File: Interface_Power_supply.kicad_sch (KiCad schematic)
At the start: 0 parts

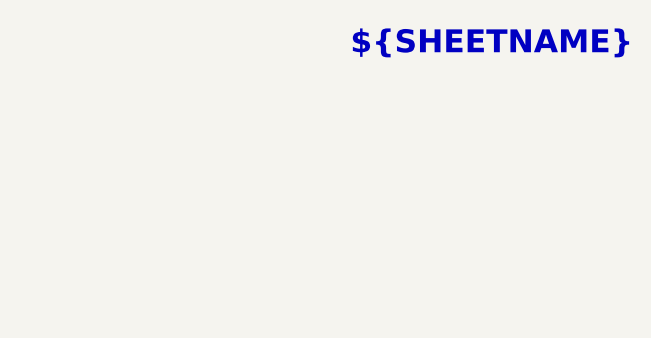
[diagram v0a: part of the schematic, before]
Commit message: testing green mask
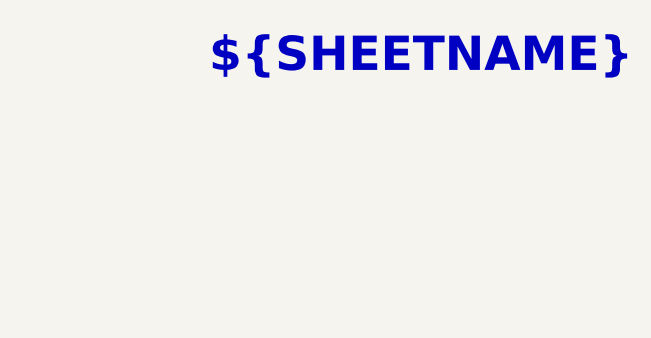
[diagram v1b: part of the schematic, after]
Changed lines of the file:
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@@
+		)
+	)
+	(text "${SHEETNAME}"
+		(exclude_from_sim no)
+		(at 283.21 14.605 0)
+		(effects
+			(font
+				(face "DejaVu Sans")
+				(size 3.81 3.81)
+				(bold yes)
+				(color 0 0 0 1)
+			)
+			(justify right top)
 		)
 	)
@@
 		)
 	)
-	(text "${SHEETNAME}"
-		(exclude_from_sim no)
-		(at 283.21 13.97 0)
-		(effects
-			(font
-				(size 2.54 2.54)
-				(bold yes)
-			)
-			(justify right top)
-		)
-	)
